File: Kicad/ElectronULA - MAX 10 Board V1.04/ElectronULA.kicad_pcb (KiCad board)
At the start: 4 copper layers, 49 x 68.4 mm, 77 parts, among them J1 Conn_01x02, J2 Micro_SD_Card_Det_Hirose_DM3AT, SW1 SW_DIP_x04, U1 10M08SCE144C8G, U10 SN74HCT125D, U2 74LVC4245APW, U3 74LVC4245APW, U4 74LVC4245APW, U5 74LVC4245APW, U6 74LVC4245APW, U7 74LVC4245APW, U8 AP111733, U9 ELECTRON_ULA_PGA_68, X1 OSC

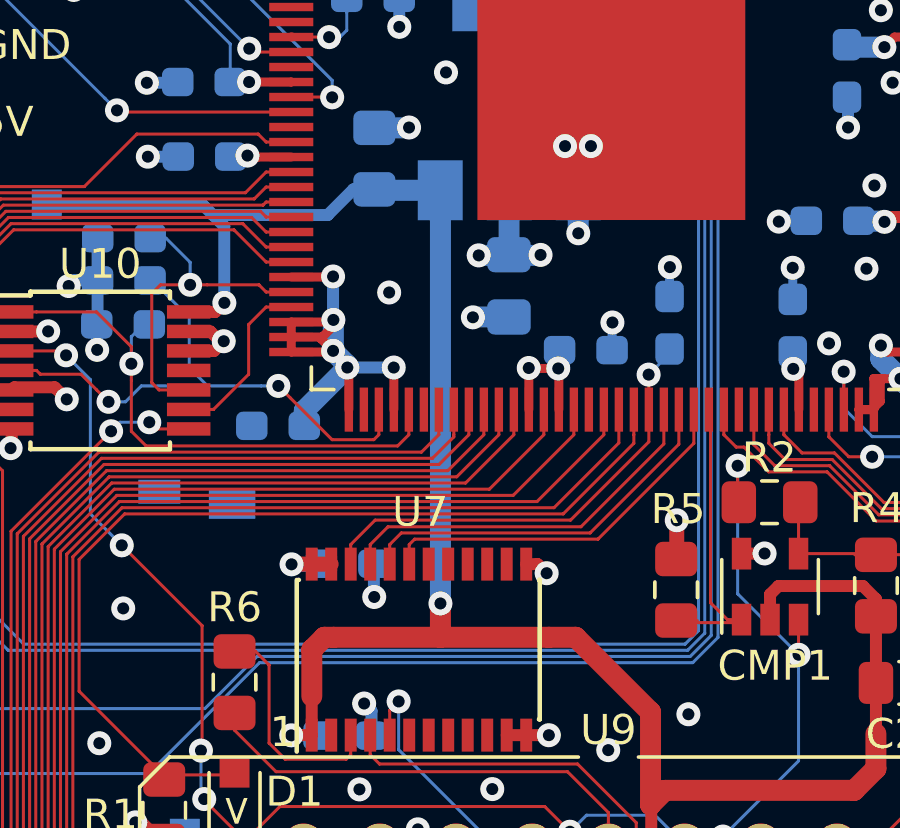
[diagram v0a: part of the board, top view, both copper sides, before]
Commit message: Updated with latest VHDL and Kicad Ver 1.05 Board
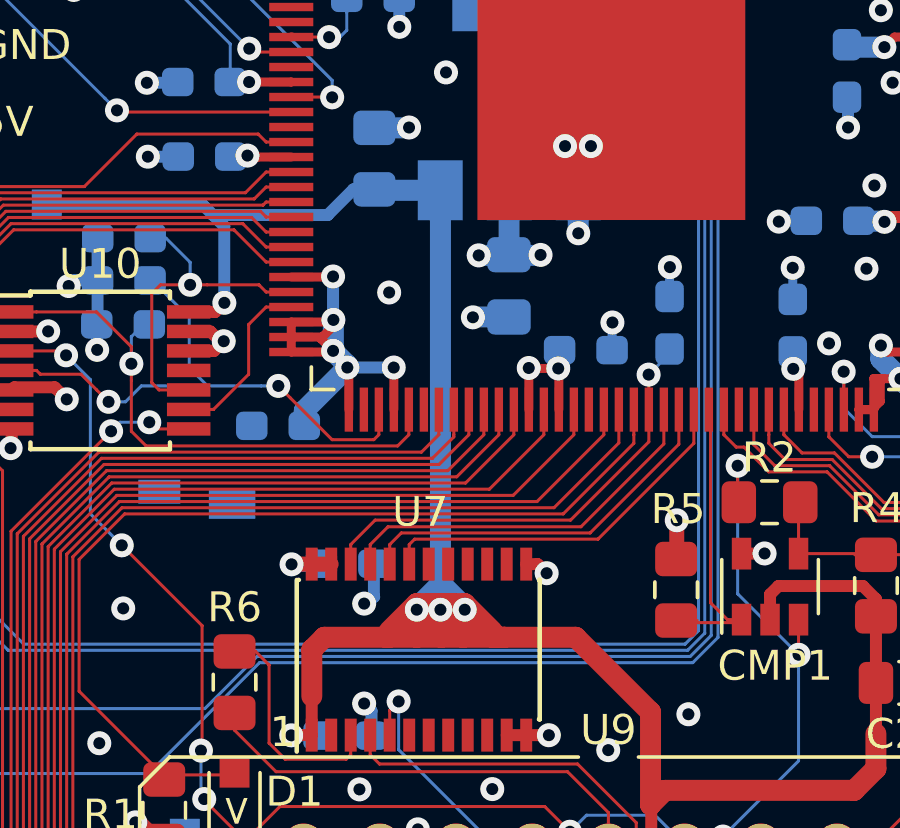
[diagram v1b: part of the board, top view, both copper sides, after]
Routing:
- net /5V: track 165.9 -> 183.3 mm, vias 9 -> 11
